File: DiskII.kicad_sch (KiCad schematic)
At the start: 31 parts, among them J1 Apple II Expansion Bus, J2 DRIVE 2, J3 DRIVE 1, Q1 2N3906, Q2 MPSU51, Q3 MPSU51, SW1 A8, SW2 A9, SW3 A10

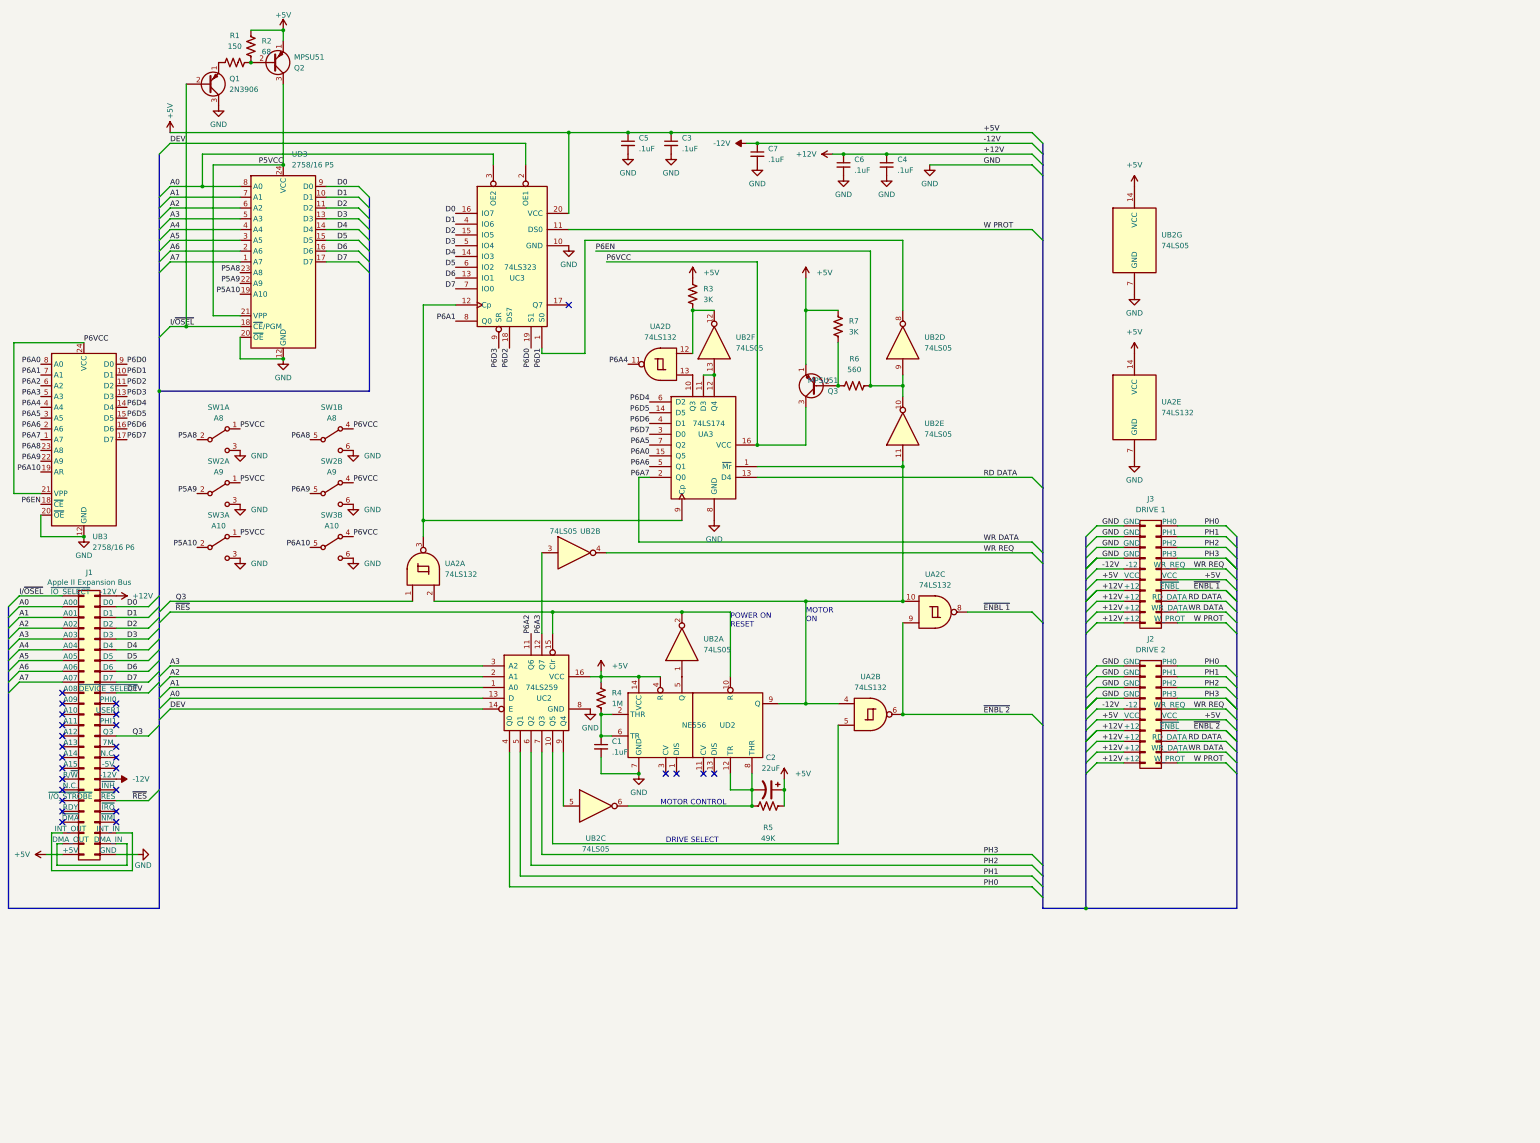
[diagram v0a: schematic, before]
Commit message: massive fixups
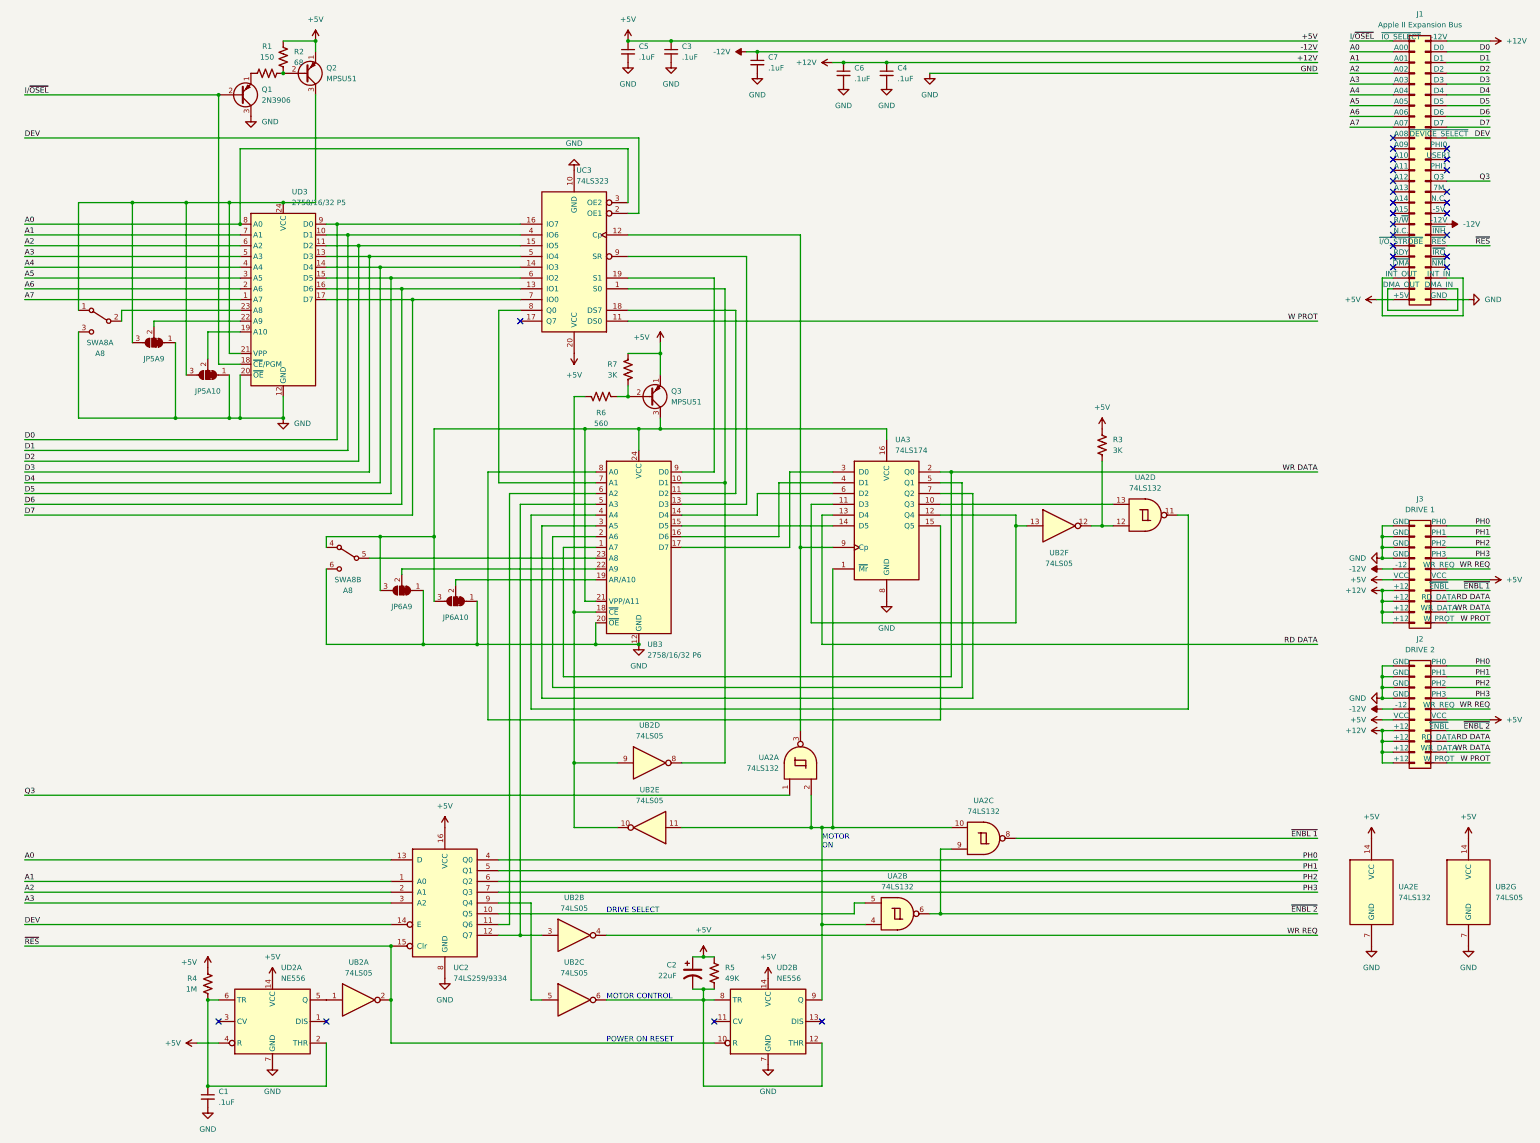
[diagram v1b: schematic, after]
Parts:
- removed SW2: A9, Connector_PinHeader_2.54mm:PinHeader_2x03_P2.54mm_Vertical, symbol Switch:SW_DPDT_x2
- removed SW3: A10, Connector_PinHeader_2.54mm:PinHeader_2x03_P2.54mm_Vertical, symbol Switch:SW_DPDT_x2
- added JP5A10, JP6A10: A10, Jumper:SolderJumper-3_P1.3mm_Bridged12_RoundedPad1.0x1.5mm_NumberLabels, symbol Jumper:SolderJumper_3_Bridged12
- added JP5A9, JP6A9: A9, Jumper:SolderJumper-3_P1.3mm_Bridged12_RoundedPad1.0x1.5mm_NumberLabels, symbol Jumper:SolderJumper_3_Bridged12
- added unit 2 of UD2
- R1, R2, R3, R6, R7: footprint Resistor_THT:R_Axial_DIN0207_L6.3mm_D2.5mm_P7.62mm_Horizontal -> Resistor_THT:R_Axial_DIN0207_L6.3mm_D2.5mm_P10.16mm_Horizontal
- R4, R5: footprint Resistor_THT:R_Axial_DIN0309_L9.0mm_D3.2mm_P12.70mm_Horizontal -> Resistor_THT:R_Axial_DIN0207_L6.3mm_D2.5mm_P10.16mm_Horizontal
- UB3: value 2758/16 P6 -> 2758/16/32 P6
- UC2: value 74LS259 -> 74LS259/9334
- UD3: value 2758/16 P5 -> 2758/16/32 P5
- renumbered SW1 to SWA8
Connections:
- net +5V: now also UD2.14 (VCC)
- net GND: now also JP5A10.1 (A), JP5A9.1 (A), JP6A10.1 (A), JP6A9.1 (A), UD2.7 (GND)
- net ~{RES}: now also UD2.10 (R); no longer UD2.10 (R)
- net at C2.2, R5.1, UB2.6: now also UD2.12 (THR), UD2.8 (TR); no longer UD2.12 (TR), UD2.8 (THR)
- net at UA2.10, UA2.2, UA2.4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: now also UD2.9 (Q); no longer UD2.9 (Q)
- net P5A10: no longer names the net of UD3.19 (A10)
- net P5A10: now also JP5A10.2 (C)
- net P5A8: no longer names the net of SWA8.2 (B), UD3.23 (A8)
- net P5A9: no longer names the net of UD3.22 (A9)
- net P5A9: now also JP5A9.2 (C)
- net P5VCC: no longer names the net of Q2.3 (C), SWA8.1 (A), UD3.21 (VPP), UD3.24 (VCC)
- net P5VCC: now also JP5A10.3 (B), JP5A9.3 (B)
- net P6A0: no longer names the net of UA3.15 (Q5), UB3.8 (A0)
- net P6A1: no longer names the net of UB3.7 (A1), UC3.8 (Q0)
- net P6A10: no longer names the net of UB3.19 (AR/A10)
- net P6A10: now also JP6A10.2 (C)
- net P6A2: no longer names the net of UB3.6 (A2), UC2.11 (Q6)
- net P6A3: no longer names the net of UB2.3, UB3.5 (A3), UC2.12 (Q7)
- net P6A4: no longer names the net of UA2.11, UB3.4 (A4)
- net P6A5: no longer names the net of UA3.7 (Q2), UB3.3 (A5)
- net P6A6: no longer names the net of UA3.5 (Q1), UB3.2 (A6)
- net P6A7 renamed WR DATA
- net P6A8: no longer names the net of SWA8.5 (B), UB3.23 (A8)
- net P6A9: no longer names the net of UB3.22 (A9)
- net P6A9: now also JP6A9.2 (C)
- net P6D0: no longer names the net of UB3.9 (D0), UC3.19 (S1)
- net P6D1: no longer names the net of UB2.8, UB3.10 (D1), UC3.1 (S0)
- net P6D2: no longer names the net of UB3.11 (D2), UC3.18 (DS7)
- net P6D3: no longer names the net of UB3.13 (D3), UC3.9 (SR)
- net P6D4: no longer names the net of UA3.6 (D2), UB3.14 (D4)
- net P6D5: no longer names the net of UA3.14 (D5), UB3.15 (D5)
- net P6D6: no longer names the net of UA3.4 (D1), UB3.16 (D6)
- net P6D7: no longer names the net of UA3.3 (D0), UB3.17 (D7)
- net P6EN: no longer names the net of R6.2, UB2.10, UB2.9, UB3.18 (~{CE})
- net P6VCC: no longer names the net of Q3.3 (C), SWA8.4 (A), UA3.16 (VCC), UB3.21 (VPP/A11), UB3.24 (VCC)
- net P6VCC: now also JP6A10.3 (B), JP6A9.3 (B)
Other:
- moved on the sheet: C2, C3, C4, C5, C6, C7, J1, J2, J3, Q1, Q2, Q3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

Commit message: revision 1
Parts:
- added JP17: Unidisk, Jumper:SolderJumper-3_P1.3mm_Bridged12_RoundedPad1.0x1.5mm, symbol Jumper:SolderJumper_3_Bridged12
- added JP19: Unidisk, Jumper:SolderJumper-2_P1.3mm_Bridged_RoundedPad1.0x1.5mm, symbol Jumper:SolderJumper_2_Bridged
- J1: value Apple II Expansion Bus -> Apple II Expansion Slot
- Q2, Q3: symbol Transistor_BJT:MPSA92 -> Device:Q_PNP_EBC
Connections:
- net +12V: now also JP17.1 (A), JP19.1 (A); no longer J3.17 (+12), J3.19 (+12)
- net ~{ENBL 2}: now also JP17.3 (B)
- new net: J3.17 (Pin_17), JP17.2 (C)
- new net: J3.19 (Pin_19), JP19.2 (B)
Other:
- moved on the sheet: C1, C2, C3, C4, C5, C6, C7, J1, J2, J3, JP5A10, JP5A9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
